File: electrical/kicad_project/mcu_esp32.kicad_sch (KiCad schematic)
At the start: 10 parts, among them J1 Conn_01x04, SW1 SW_Push, SW2 SW_Push, U2 ESP32-WROOM-32

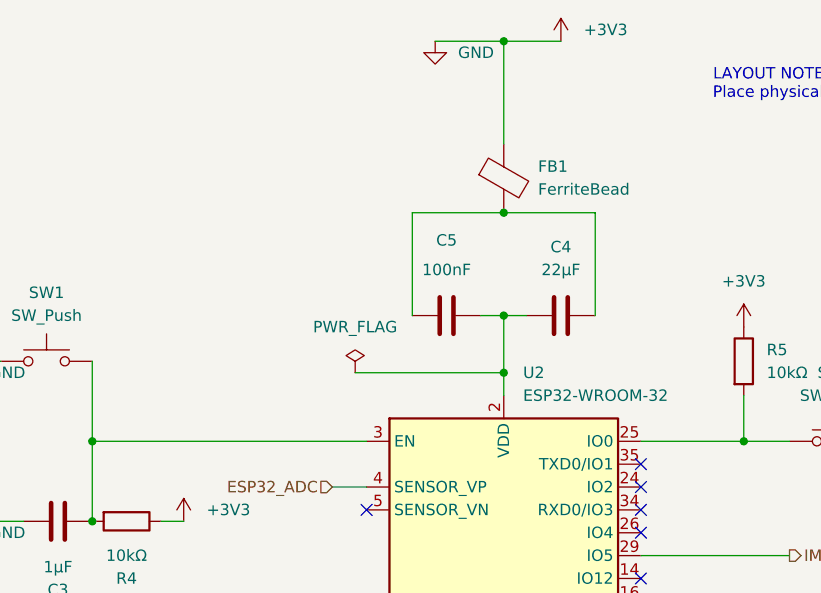
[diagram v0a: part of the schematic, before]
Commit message: new push
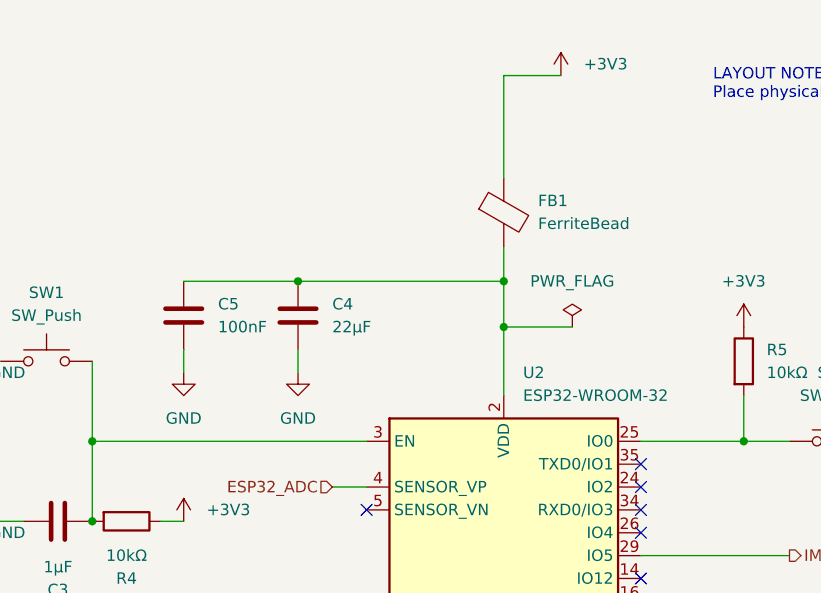
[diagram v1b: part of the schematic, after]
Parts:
- C3, C5: footprint (none) -> Capacitor_SMD:C_0402_1005Metric
- C4: footprint (none) -> Capacitor_SMD:C_0805_2012Metric
- FB1: footprint (none) -> Inductor_SMD:L_0402_1005Metric
- J1: footprint (none) -> Connector_JST:JST_SH_SM04B-SRSS-TB_1x04-1MP_P1.00mm_Horizontal
- R4, R5: footprint (none) -> Resistor_SMD:R_0402_1005Metric
- SW1, SW2: footprint (none) -> Button_Switch_SMD:SW_SPST_B3U-1000P
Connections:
- net +3V3: no longer C3.2, J1.4 (Pin_4), SW1.1, SW2.2, U2.1 (GND), U2.15 (GND), U2.38 (GND), U2.39 (GND)
- net at C5.1, U2.2 (VDD): now also C4.1, FB1.2; no longer C4.2
- new net GND: C3.2, C4.2, C5.2, J1.4 (Pin_4), SW1.1, SW2.2, U2.1 (GND), U2.15 (GND), U2.38 (GND), U2.39 (GND)
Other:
- moved on the sheet: C4, C5, FB1
